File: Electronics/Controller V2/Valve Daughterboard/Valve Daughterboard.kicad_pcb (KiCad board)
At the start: 2 copper layers, 62 x 69.5 mm, 25 parts, among them J1 Conn_01x08, J10 Conn_01x10, J11 Conn_01x02, J12 Conn_01x02, J13 Conn_01x02, J14 Conn_01x02, J15 Conn_01x02, J16 Conn_01x02, J17 Conn_01x02, J18 Conn_01x02, J19 Conn_01x08, J2 Conn_01x02, J20 Conn_01x10, J3 Conn_01x02, J4 Conn_01x02, J5 Conn_01x02, J6 Conn_01x02, J7 Conn_01x02, J8 Conn_01x02, J9 Conn_01x02

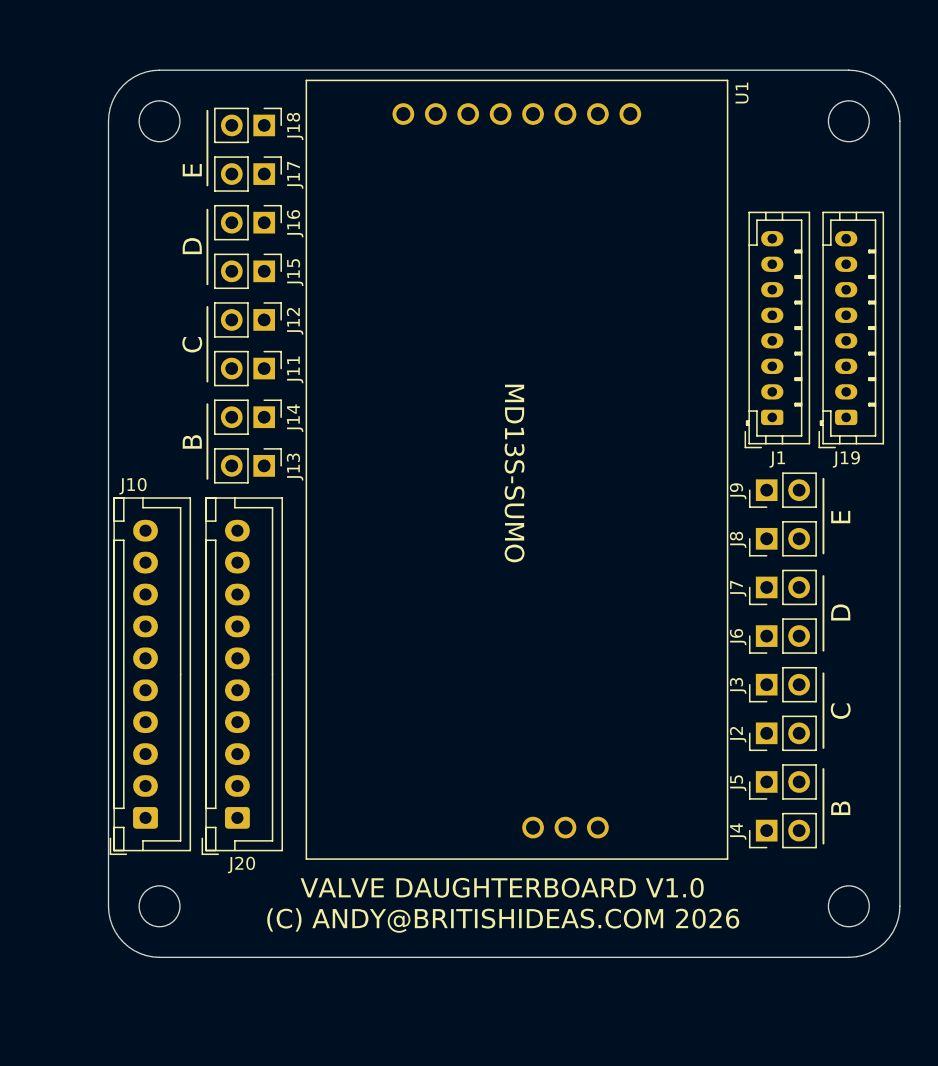
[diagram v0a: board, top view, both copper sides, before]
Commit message: Completed daughterboards.
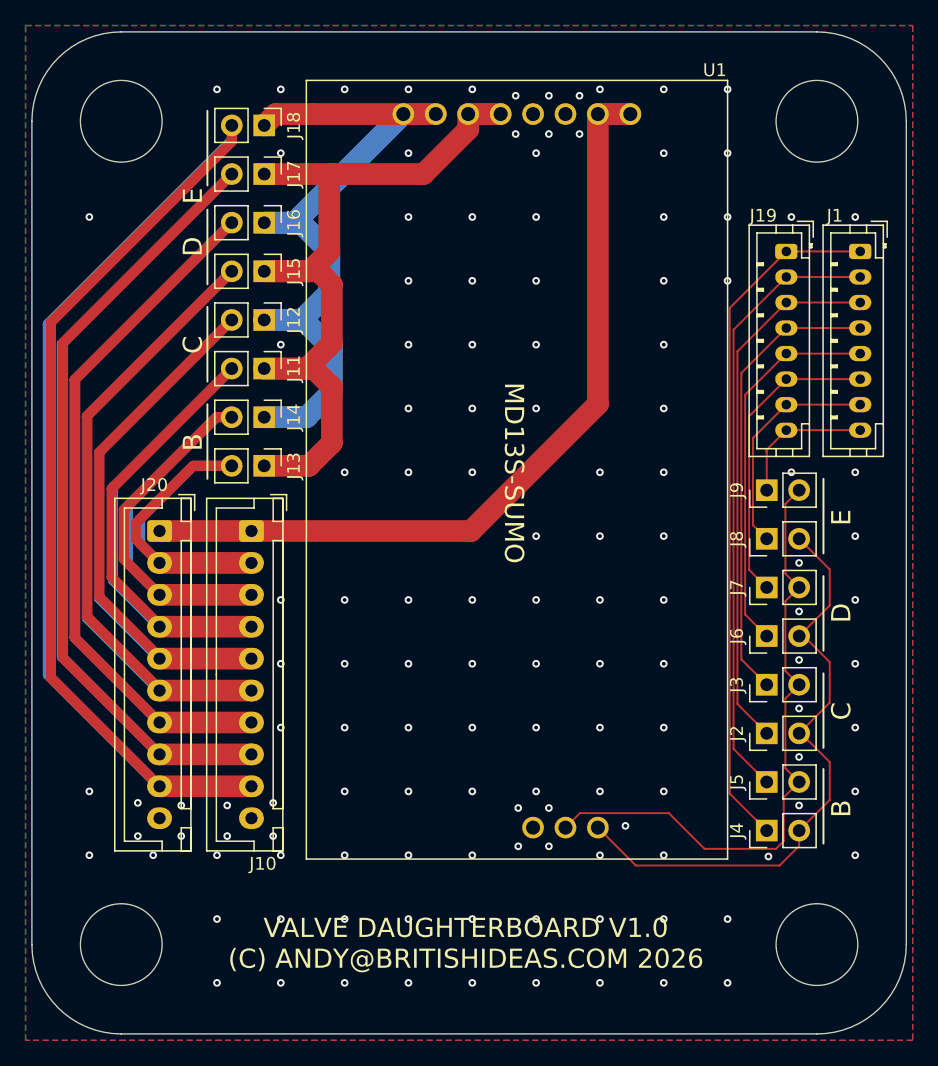
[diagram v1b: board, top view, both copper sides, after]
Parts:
- H1, H2, H3, H4: footprint MountingHole:MountingHole_3.2mm_M3 -> MountingHole:MountingHole_6.4mm_M6
- moved J10 24.0 mm to (98.7, 92.1), turned to -90 degrees
- moved J20 23.3 mm to (91.5, 92.1), turned to -90 degrees
- moved J1 14.7 mm to (146.4, 70.2), turned to -90 degrees
- moved J19 13.8 mm to (140.6, 70.2), turned to -90 degrees
- moved H3 4.24 mm to (88.5, 124.5)
- moved H4 3.91 mm to (143.0, 124.5)
- moved H1 3.00 mm to (88.5, 60.0)
- moved H2 2.50 mm to (143.0, 60.0)
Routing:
- net /VALVE_E_MB: track 0.00 -> 129.7 mm
- net /VALVE_E_MA: track 0.00 -> 115.4 mm
- net /VALVE_D_MB: track 0.00 -> 101.2 mm
- net /VALVE_D_MA: track 0.00 -> 87.0 mm
- net /VALVE_C_MB: track 0.00 -> 72.8 mm
- net Net-(J11-Pin_1): track 0.00 -> 68.4 mm
- net +12V: track 0.00 -> 66.3 mm
- net Net-(J12-Pin_1): track 0.00 -> 61.8 mm
- net /VALVE_C_MA: track 0.00 -> 58.5 mm
- net /VALVE_B_DIR: track 0.00 -> 54.2 mm
- net Net-(J3-Pin_2): track 0.00 -> 49.7 mm
- net /VALVE_B_PWM: track 0.00 -> 48.1 mm
- net Net-(J2-Pin_2): track 0.00 -> 47.9 mm
- net /VALVE_B_MB: track 0.00 -> 45.5 mm
- net /VALVE_C_DIR: track 0.00 -> 42.1 mm
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- added copper zone on B.Cu, net GND
- added copper zone on F.Cu, net GND
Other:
- board size 62 x 69.5 mm -> 68.5 x 78.5 mm
